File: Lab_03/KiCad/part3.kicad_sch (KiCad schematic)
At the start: 22 parts, among them Q301 NMOS, U301 LM324, U302 LM339

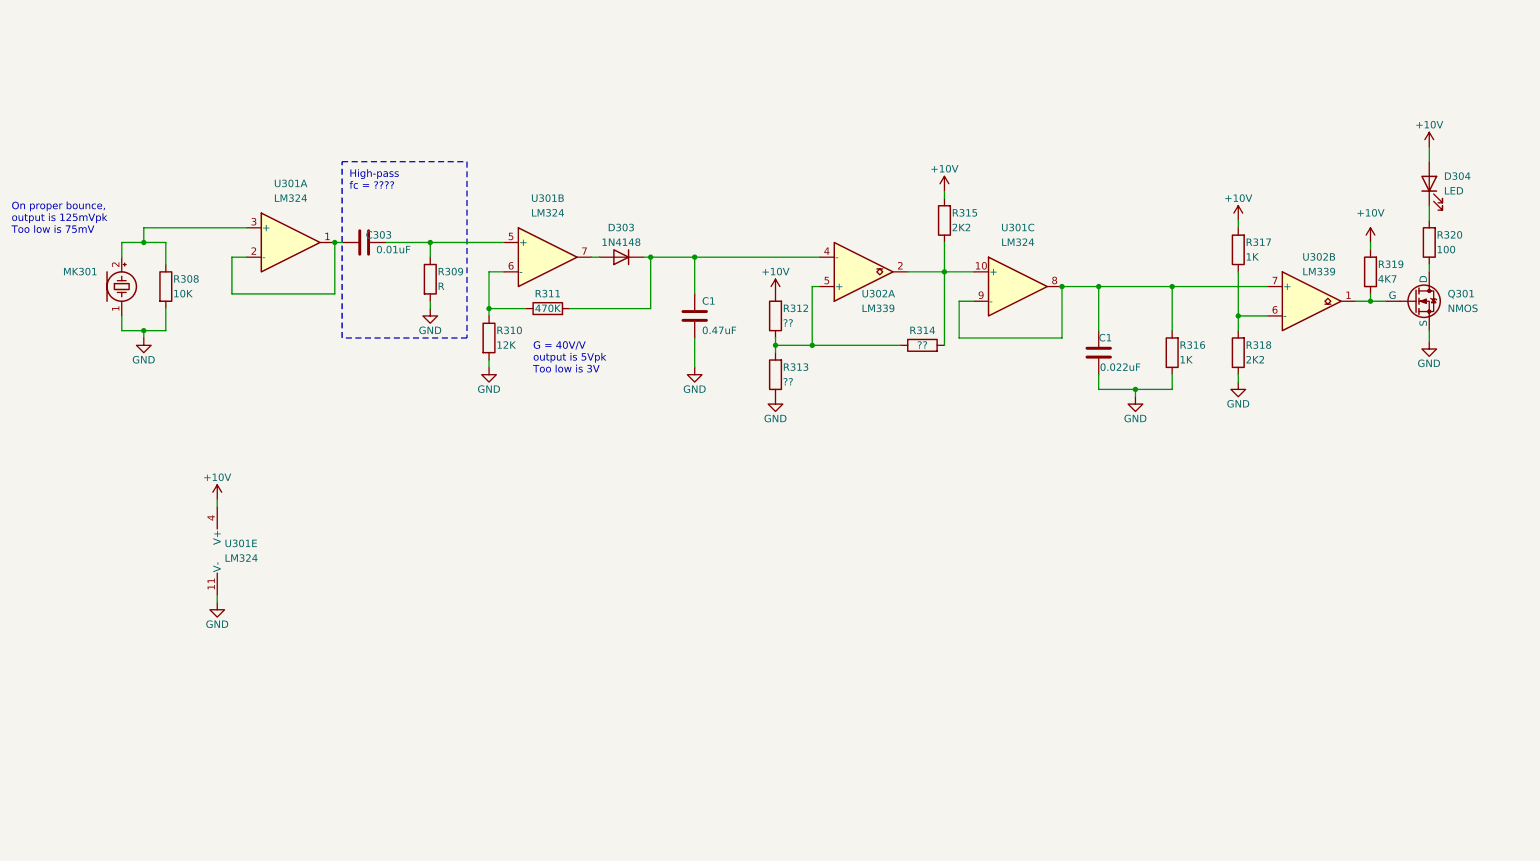
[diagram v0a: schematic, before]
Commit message: final lab3
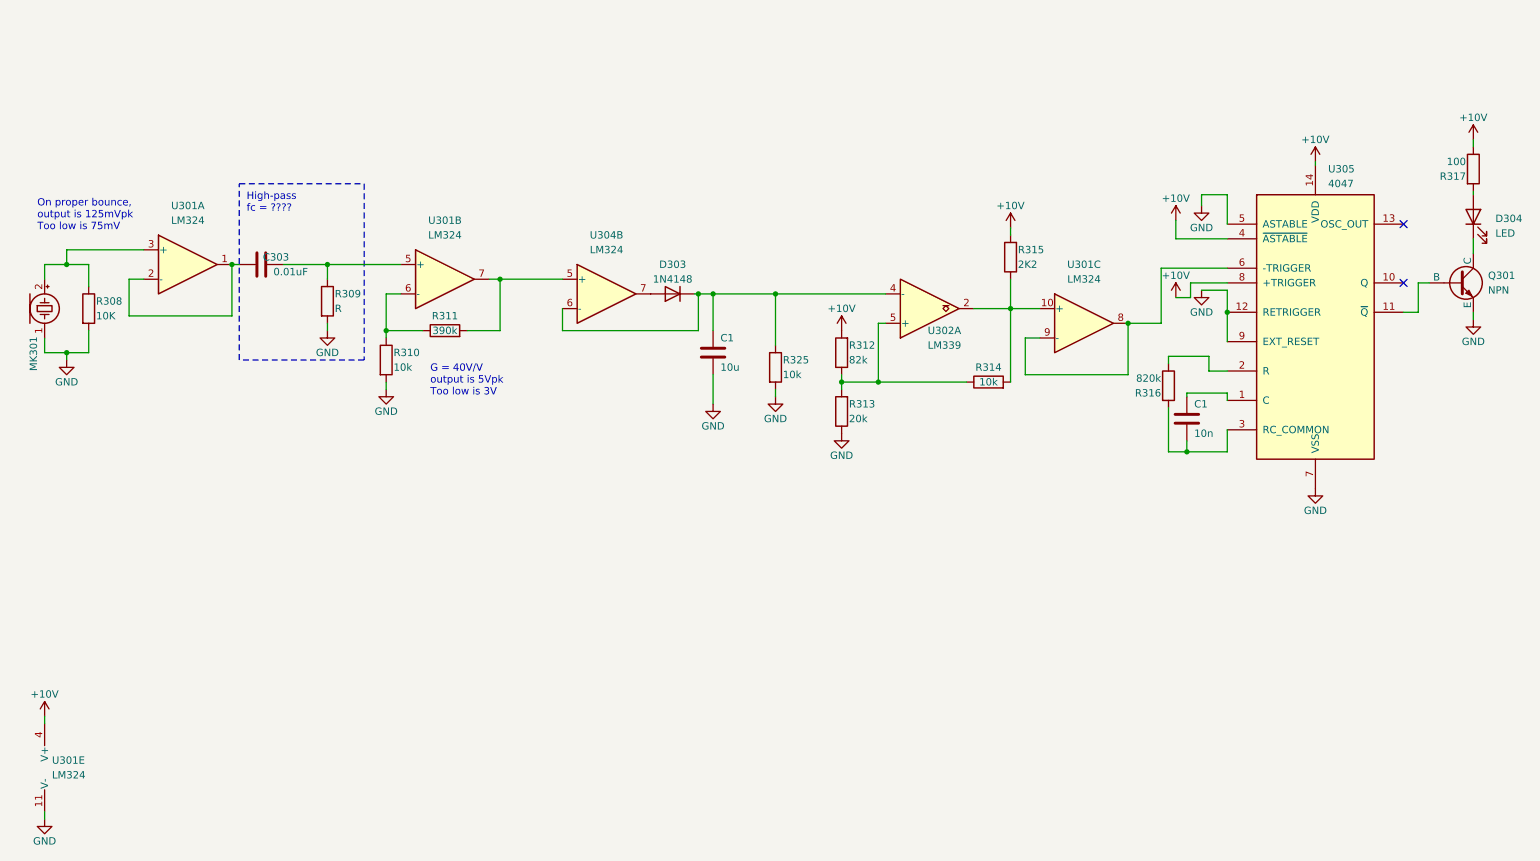
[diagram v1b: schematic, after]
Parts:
- removed C1: 0.47uF, symbol Device:C
- removed C1: 0.022uF, symbol Device:C
- removed Q301: NMOS, symbol Simulation_SPICE:NMOS
- removed R318: 2K2, symbol Device:R
- removed R319: 4K7, symbol Device:R
- removed R320: 100, symbol Device:R
- removed unit 2 of U302
- added C1: 10u, symbol Device:C
- added C1: 10n, symbol Device:C
- added Q301: NPN, symbol Simulation_SPICE:NPN
- added R325: 10k, symbol Device:R
- added U304: LM324, symbol Amplifier_Operational:LM324
- added U305: 4047, symbol 4xxx:4047
- R310: value 12K -> 10k
- R311: value 470K -> 390k
- R312: value ?? -> 82k
- R313: value ?? -> 20k
- R314: value ?? -> 10k
- R316: value 1K -> 820k
- R317: value 1K -> 100
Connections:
- net +10V: now also R317.1, U305.14 (VDD), U305.4 (~{ASTABLE}), U305.8 (+TRIGGER); no longer D304.2 (A), R317.2
- net GND: now also C1.1, Q301.3 (E), R325.2, U305.12 (RETRIGGER), U305.5 (ASTABLE), U305.7 (VSS), U305.9 (EXT_RESET); no longer R316.1
- net at D304.1 (K): now also Q301.1 (C)
- net at D303.1 (K), U302.4 (-): now also C1.2, R325.1, U304.6 (-); no longer R311.2
- net at U301.8, U301.9 (-): now also U305.6 (-TRIGGER); no longer R316.2
- net at U301.7: now also R311.2, U304.5 (+); no longer D303.2 (A)
- new net: C1.2, U305.1 (C)
- new net: Q301.2 (B), U305.11 (~{Q})
- new net: R316.1, U305.2 (R)
- new net: C1.1, R316.2, U305.3 (RC_COMMON)
- new net: D303.2 (A), U304.7
- new net: D304.2 (A), R317.2
- no-connect marks 0 -> 2
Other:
- moved on the sheet: C303, MK301, R308, R309, R310, R311, R312, R313, R314, R315, U301A, U301B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

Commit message: Finalize Lab 3 Post-Recitation
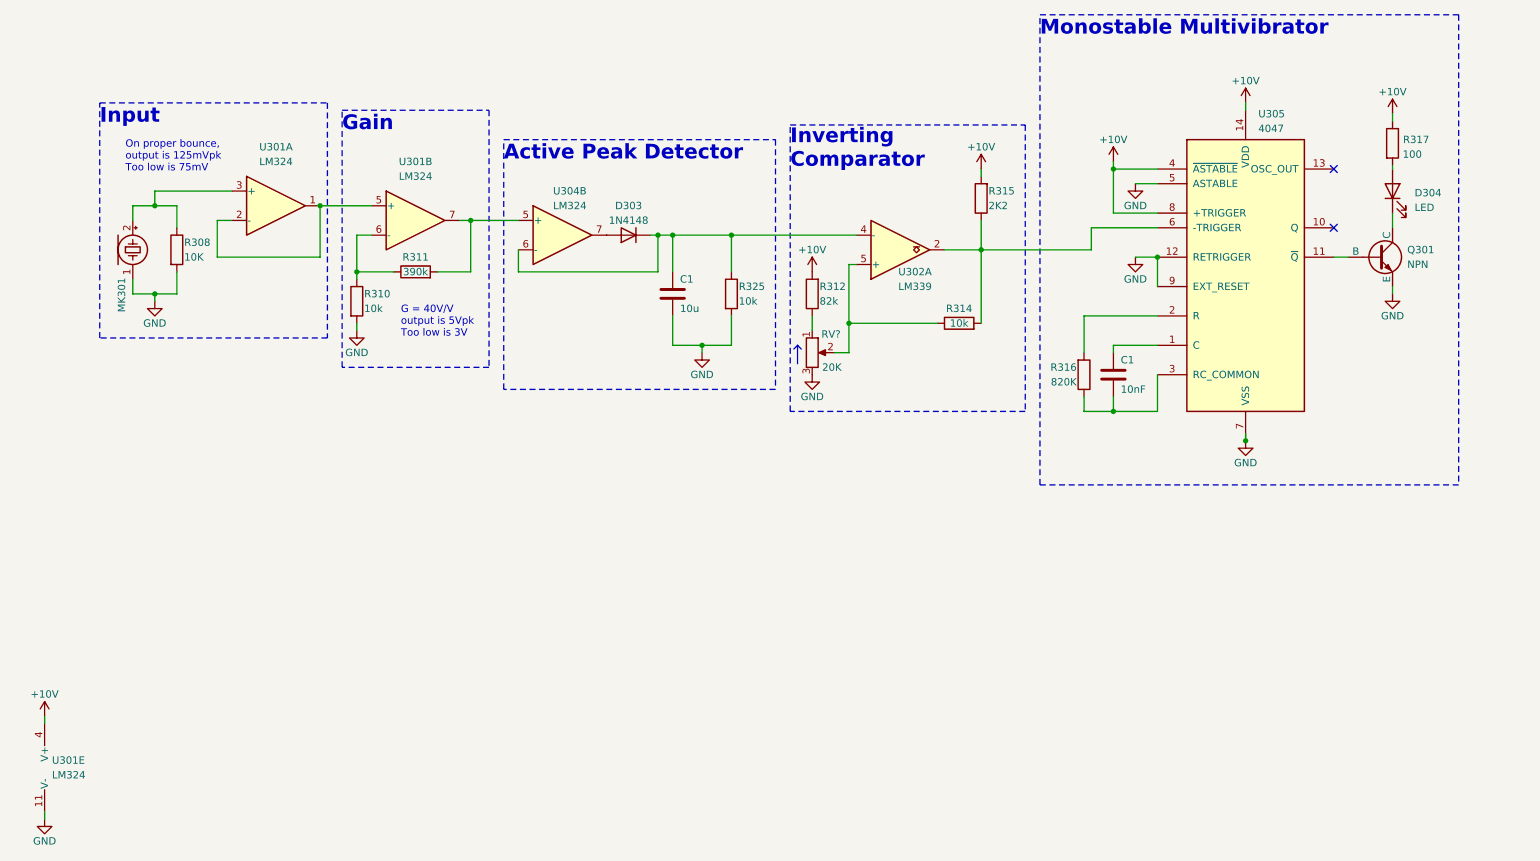
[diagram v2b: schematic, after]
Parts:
- removed C303: 0.01uF, symbol Device:C
- removed R309: R, symbol Device:R
- removed R313: 20k, symbol Device:R
- removed unit 3 of U301
- added RV?: 20K, symbol Device:R_Potentiometer
- C1: value 10n -> 10nF
- R316: value 820k -> 820K
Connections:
- net GND: now also RV?.3
- net at R314.1, U302.5 (+): now also RV?.2; no longer R312.1
- net at R314.2, R315.1, U302.2: now also U305.6 (-TRIGGER)
- net at U301.1, U301.2 (-): now also U301.5 (+)
- net at U305.2 (R): now also R316.2; no longer R316.1
- net at C1.1, U305.3 (RC_COMMON): now also R316.1; no longer R316.2
- new net: R312.1, RV?.1
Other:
- note added: "Active Peak Detector"
- note added: "Gain"
- note added: "Input"
- note added: "Inverting Comparator"
- note added: "Monostable Multivibrator"
- note removed: "High-pass fc = ????"
- moved on the sheet: C1, D303, D304, MK301, Q301, R308, R310, R311, R312, R314, R315, R316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
